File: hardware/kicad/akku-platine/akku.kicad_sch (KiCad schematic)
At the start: 22 parts, among them J1 JST PH 5-polig, J2 Strommessung, Q1 FS8205, Q2 AO3400A, Q3 AO3400A, U1 HY2111-GB, U2 TMP390A2DRL, U3 TMP390A2DRL

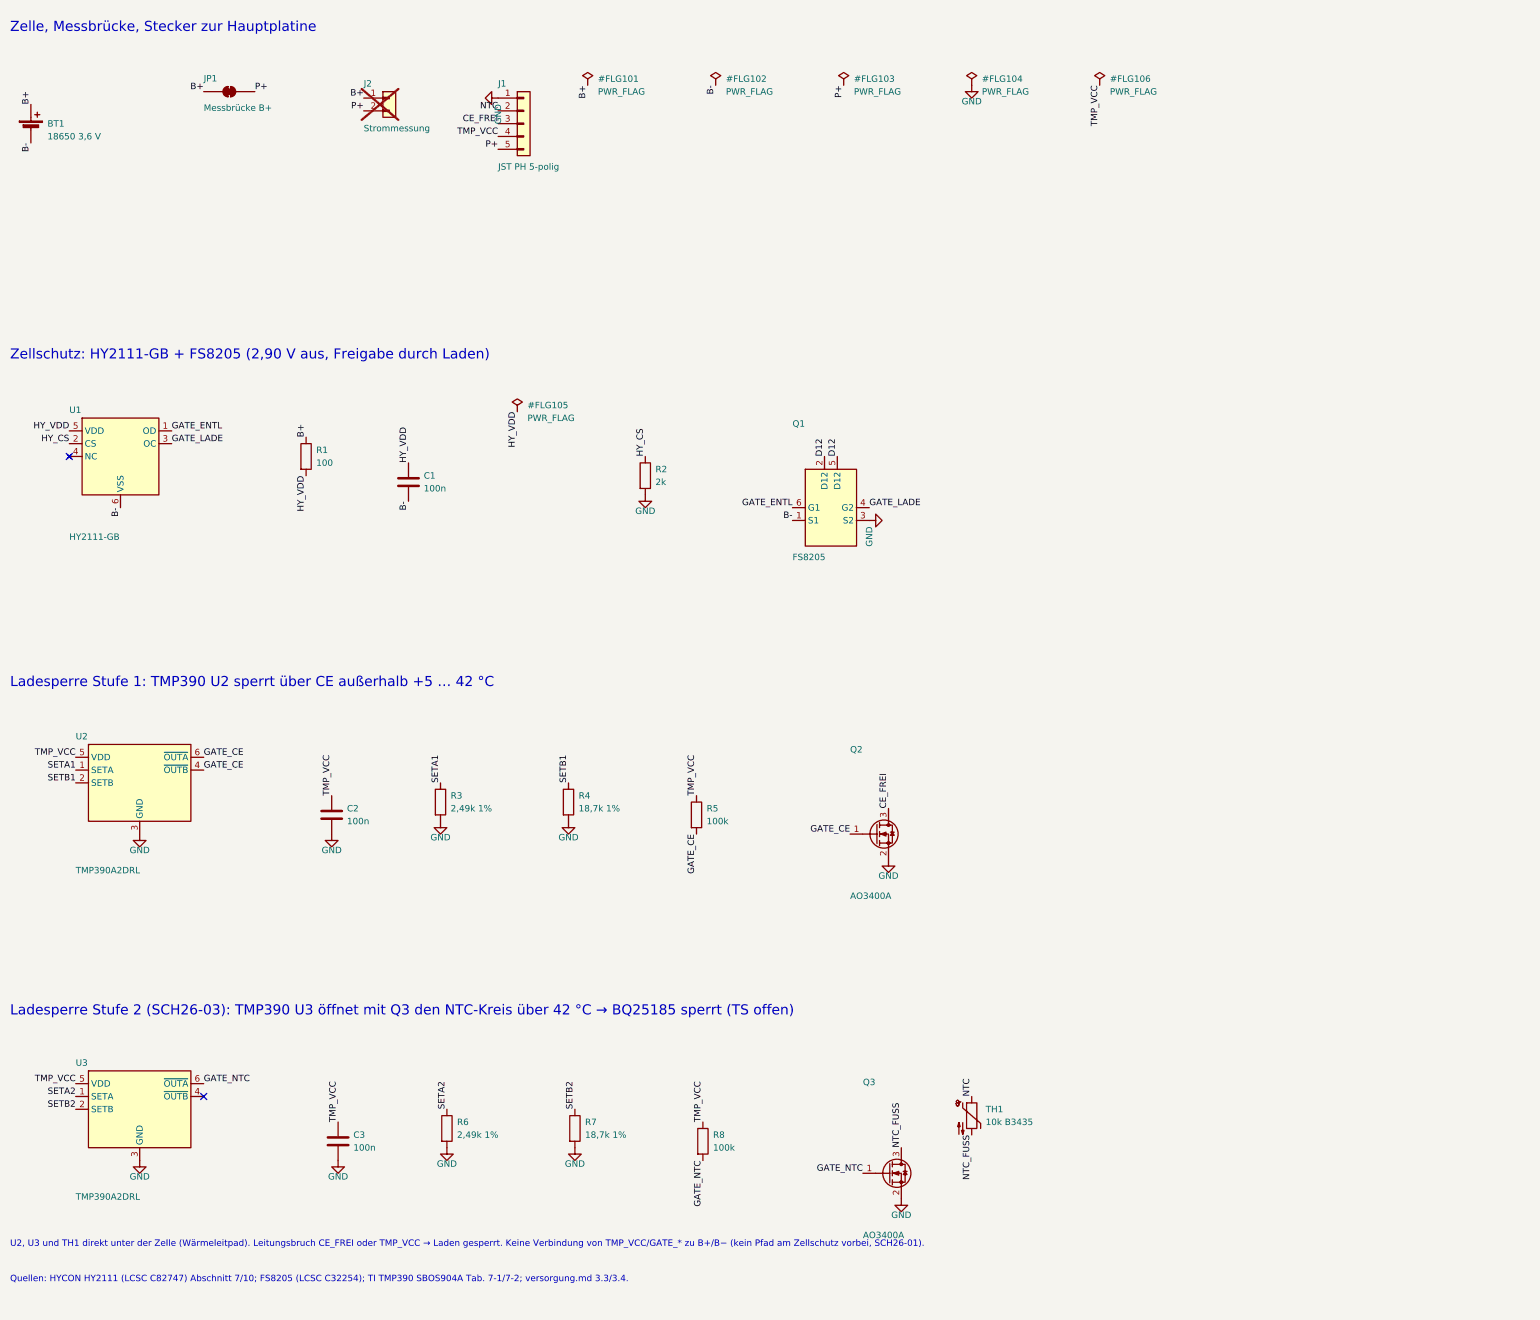
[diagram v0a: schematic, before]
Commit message: update
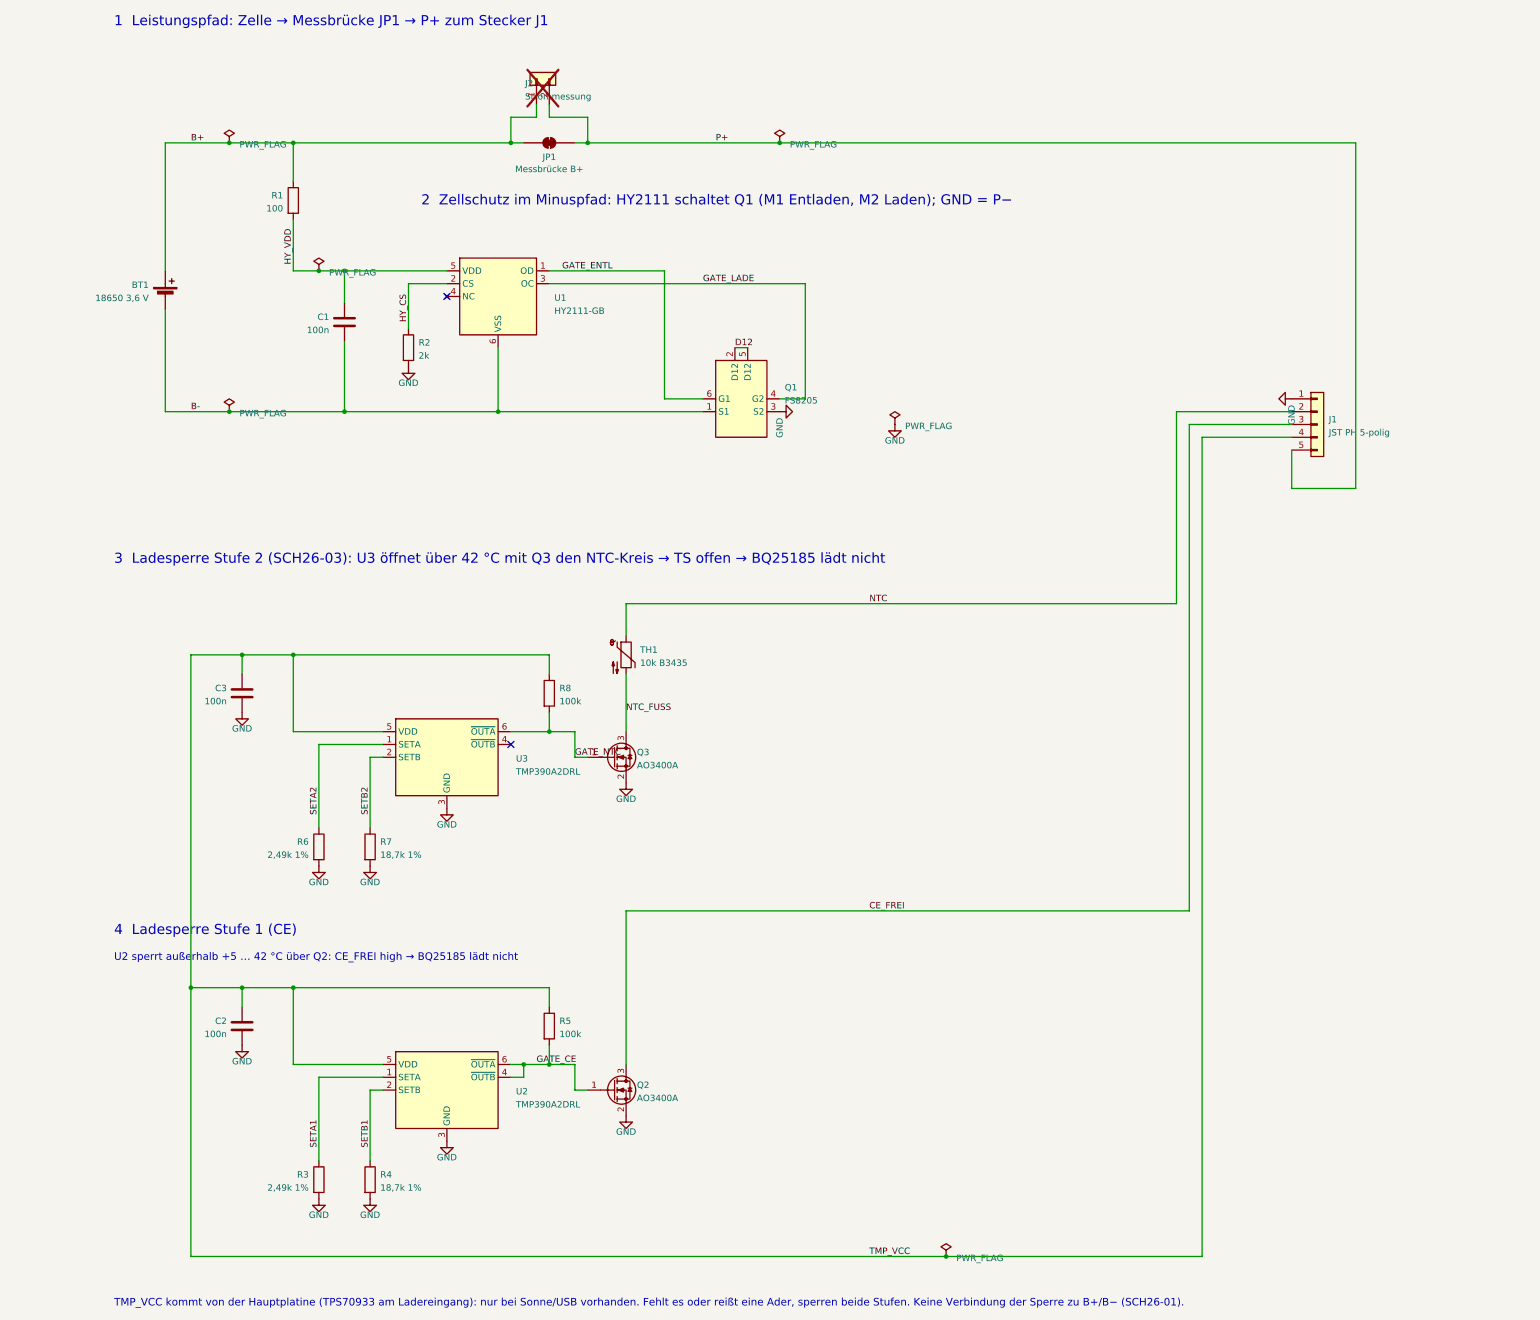
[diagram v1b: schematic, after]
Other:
- note added: "1 Leistungspfad: Zelle → Messbrücke JP1 → P+ zum Stecker J1"
- note added: "2 Zellschutz im Minuspfad: HY2111 schaltet Q1 (M1 Entladen, M2 Laden); GND = P−"
- note added: "3 Ladesperre Stufe 2 (SCH26-03): U3 öffnet über 42 °C mit Q3 den NTC-Kreis → TS offen → BQ25185 lädt nicht"
- note added: "4 Ladesperre Stufe 1 (CE)"
- note added: "TMP_VCC kommt von der Hauptplatine (TPS70933 am Ladereingang): nur bei Sonne/USB vorhanden. Fehlt es oder reißt eine Ader, sperren beide Stufen. Keine Verbindung der Sperre zu B+/B− (SCH26-01)."
- note added: "U2 sperrt außerhalb +5 … 42 °C über Q2: CE_FREI high → BQ25185 lädt nicht"
- note removed: "Ladesperre Stufe 1: TMP390 U2 sperrt über CE außerhalb +5 … 42 °C"
- note removed: "Ladesperre Stufe 2 (SCH26-03): TMP390 U3 öffnet mit Q3 den NTC-Kreis über 42 °C → BQ25185 sperrt (TS offen)"
- note removed: "Quellen: HYCON HY2111 (LCSC C82747) Abschnitt 7/10; FS8205 (LCSC C32254); TI TMP390 SBOS904A Tab. 7-1/7-2; versorgung.md 3.3/3.4."
- note removed: "U2, U3 und TH1 direkt unter der Zelle (Wärmeleitpad). Leitungsbruch CE_FREI oder TMP_VCC → Laden gesperrt. Keine Verbindung von TMP_VCC/GATE_* zu B+/B− (kein Pfad am Zellschutz vorbei, SCH26-01)."
- note removed: "Zelle, Messbrücke, Stecker zur Hauptplatine"
- note removed: "Zellschutz: HY2111-GB + FS8205 (2,90 V aus, Freigabe durch Laden)"
- moved on the sheet: BT1, C1, C2, C3, J1, J2, JP1, Q1, Q2, Q3, R1, R2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

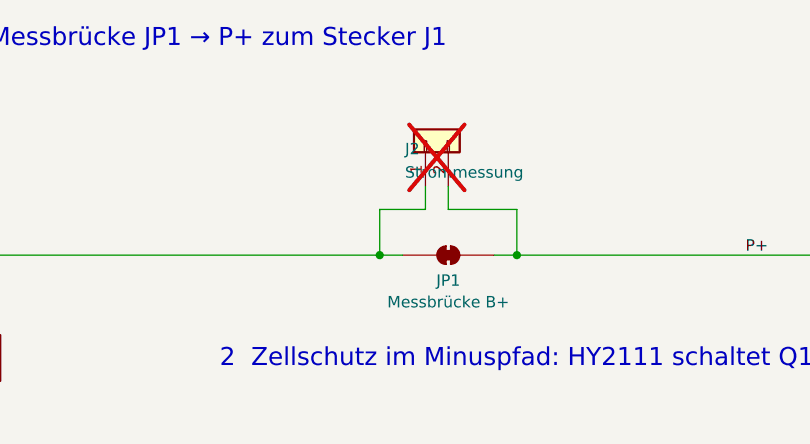
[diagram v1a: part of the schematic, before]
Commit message: Wetter-Eingang hinzugefügt
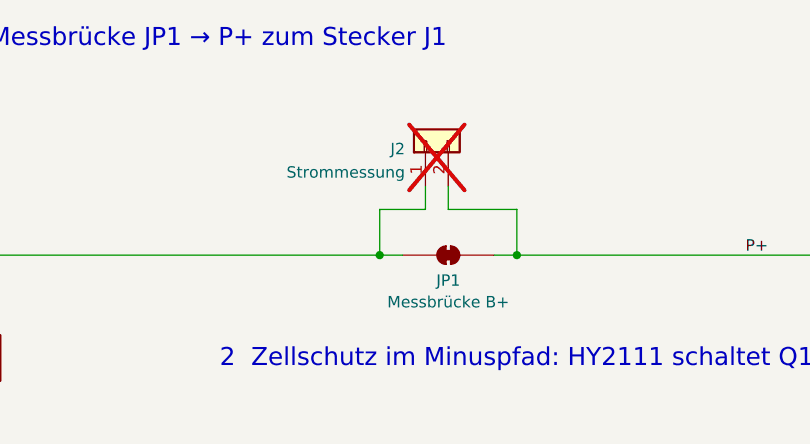
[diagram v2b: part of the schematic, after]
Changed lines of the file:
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@@
 					(size 1.27 1.27)
 				)
-				(justify right)
+				(justify left)
 			)
 		)
@@
 					(size 1.27 1.27)
 				)
-				(justify right)
+				(justify left)
 			)
 		)
